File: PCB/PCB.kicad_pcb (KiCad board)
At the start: 2 copper layers, 31 parts, among them SW1 Bourns PEC11R, SW2 Bourns PEC11R, U1 RPi_Pico_TH, U2 RDA5807M_Module, U3 LM386, U4 AP63205WU-7

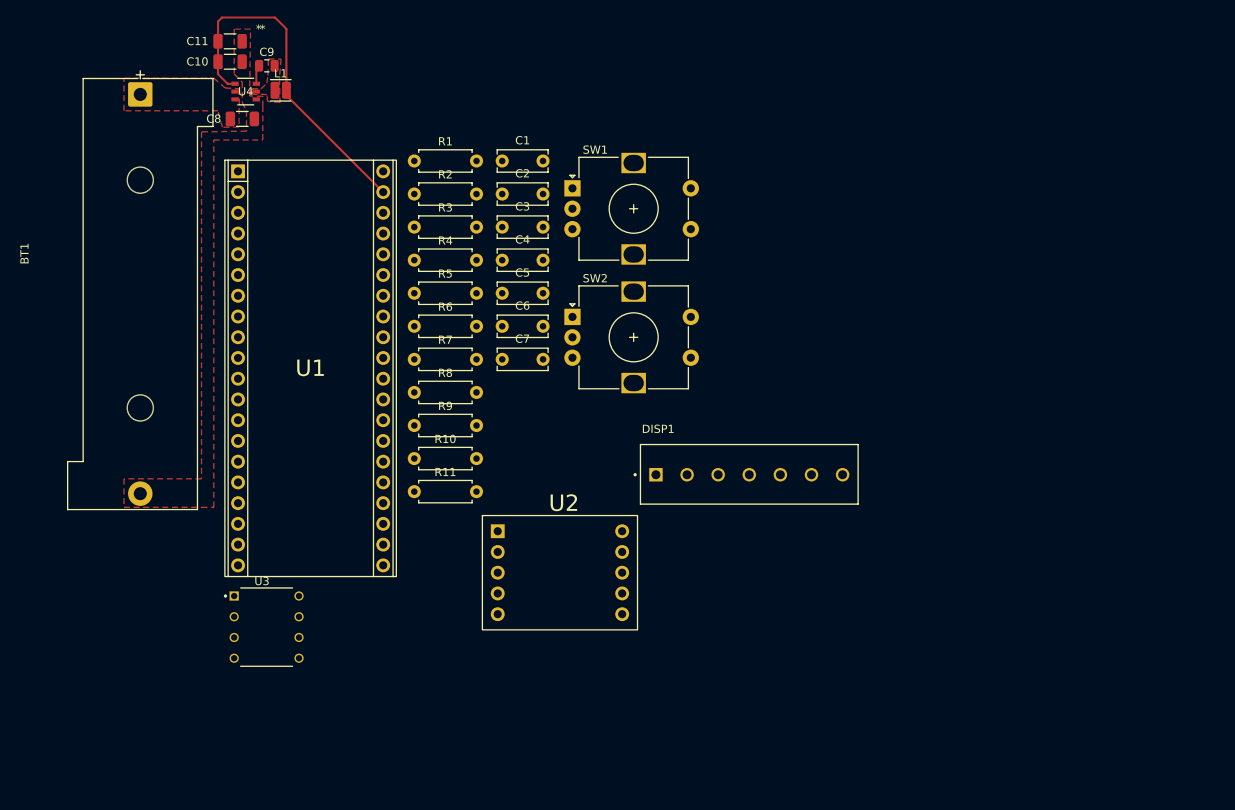
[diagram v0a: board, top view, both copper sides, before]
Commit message: PCB design #1
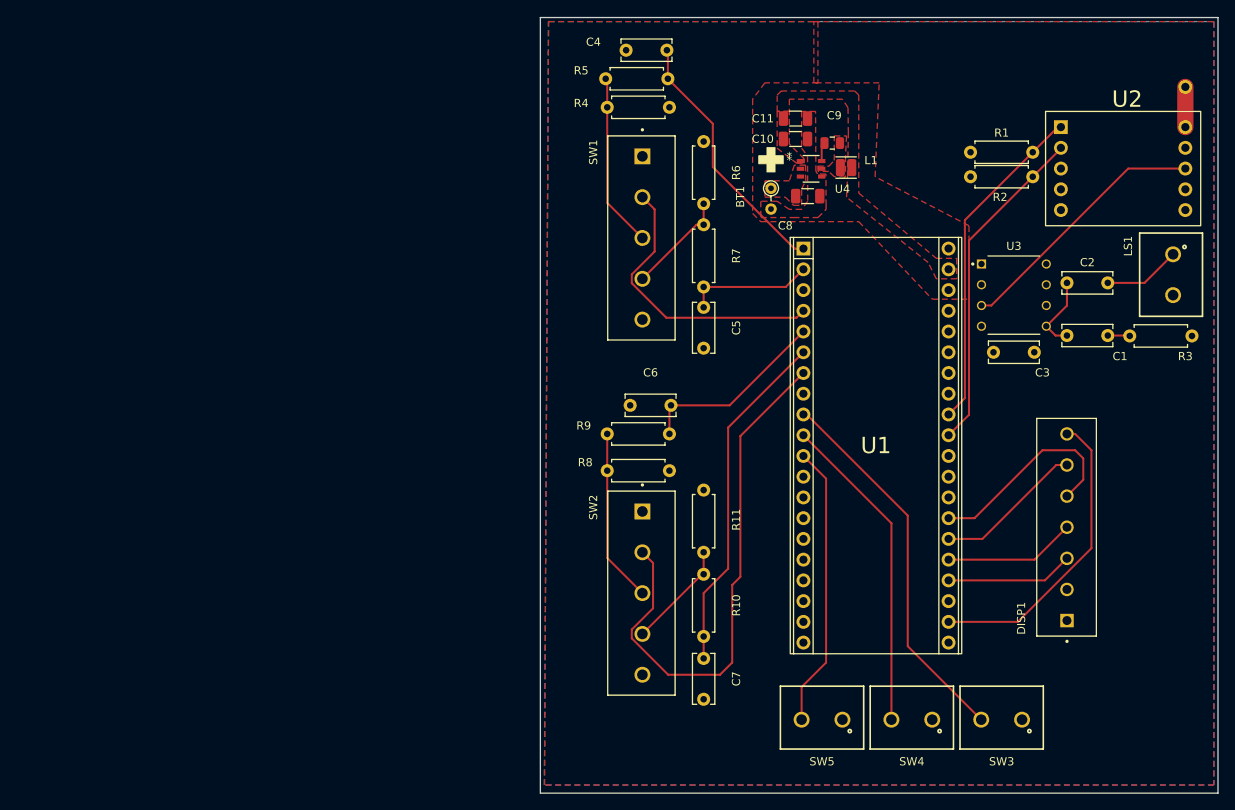
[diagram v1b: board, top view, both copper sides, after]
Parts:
- added ?: , , F.Cu at (179.0, 53.5)
- added LS1: Speaker, 2pin_ScrewTerminal:691137710002, F.Cu at (177.5, 76.5)
- added SW3: SW_DPST, 2pin_ScrewTerminal:691137710002, F.Cu at (156.5, 131.0)
- added SW4: SW_DPST, 2pin_ScrewTerminal:691137710002, F.Cu at (145.5, 131.0)
- added SW5: SW_DPST, 2pin_ScrewTerminal:691137710002, F.Cu at (134.5, 131.0)
- BT1: footprint Battery:BatteryHolder_Bulgin_BX0034_1xAAA -> Battery:THT Battery Connection
- SW1, SW2: footprint Rotary_Encoder:RotaryEncoder_Alps_EC12E-Switch_Vertical_H20mm -> 5pin_ScrewTerminal:PHOENIX_1935190
- moved U3 100.2 mm to (158.0, 79.0)
- moved R3 88.6 mm to (172.2, 84.0)
- moved U2 84.9 mm to (171.4, 63.5)
- moved BT1 78.1 mm to (128.2, 65.9)
- moved C1 72.4 mm to (164.5, 84.0)
- moved C2 70.0 mm to (164.5, 77.5)
- moved U1 69.9 mm to (141.1, 97.4)
- moved C10 69.9 mm to (131.2, 59.9)
- moved C11 69.9 mm to (131.2, 57.4)
- moved C8 69.9 mm to (132.8, 66.9)
- moved C9 69.9 mm to (135.8, 60.4)
- moved U4 69.9 mm to (133.2, 63.5)
- moved L1 69.9 mm to (137.4, 63.4)
- moved R2 68.2 mm to (152.7, 64.5)
- moved R1 68.1 mm to (152.7, 61.5)
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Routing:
- net /Encoder2SW: track 0.00 -> 66.0 mm
- net /B1: track 0.00 -> 46.7 mm
- net /Encoder2B: track 0.00 -> 42.6 mm
- net Net-(U1-VSYS): track 43.1 -> 0.61 mm
- net /Radio sdio: track 0.00 -> 41.1 mm
- net /Radio sclk: track 0.00 -> 40.9 mm
- net /B2: track 0.00 -> 39.3 mm
- net /Display CS: track 0.00 -> 37.1 mm
- net /Encoder1SW: track 0.00 -> 35.4 mm
- net /B3: track 0.00 -> 34.7 mm
- net Net-(U2-LOUT): track 0.00 -> 31.9 mm
- net /Encoder1A: track 0.00 -> 31.9 mm
- net /Display res: track 0.00 -> 25.8 mm
- net /Encoder2A: track 0.00 -> 23.5 mm
- net Net-(R4-Pad2): track 0.00 -> 21.4 mm
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- added copper zone on F.Cu, net 3V3
- added copper zone on B.Cu, net GND
- added copper zone on F.Cu, net GND
- added copper zone on F.Cu, net Net-(BT1-+)
- added copper zone on F.Cu, net Net-(U1-VSYS)
- added copper zone on F.Cu, net Net-(U4-SW)
- removed copper zone on F.Cu, net (none)
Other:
- board outline added: 83 x 95 mm
